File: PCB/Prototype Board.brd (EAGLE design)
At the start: 55.9 x 76.2 mm, 71 parts, among them IC1 SMF05CT1G, J1 USB Type C, J3 Connector, Q1 S8050, Q10 20V/0.2A/8MHz/1.2Ω/1Vth, Q2 20V/0.2A/8MHz/1.2Ω/1Vth, Q3 20V/4.2A/52mΩ/1.4W, Q4 S8050, Q5 20V/0.2A/8MHz/1.2Ω/1Vth, Q6 20V/0.2A/8MHz/1.2Ω/1Vth, Q7 20V/0.2A/8MHz/1.2Ω/1Vth, Q8 20V/0.2A/8MHz/1.2Ω/1Vth, U1 9DoF IMU, U2 MCP73831, U3 ESP-WROOM-32, U5 DWM1000, U7 CH340C

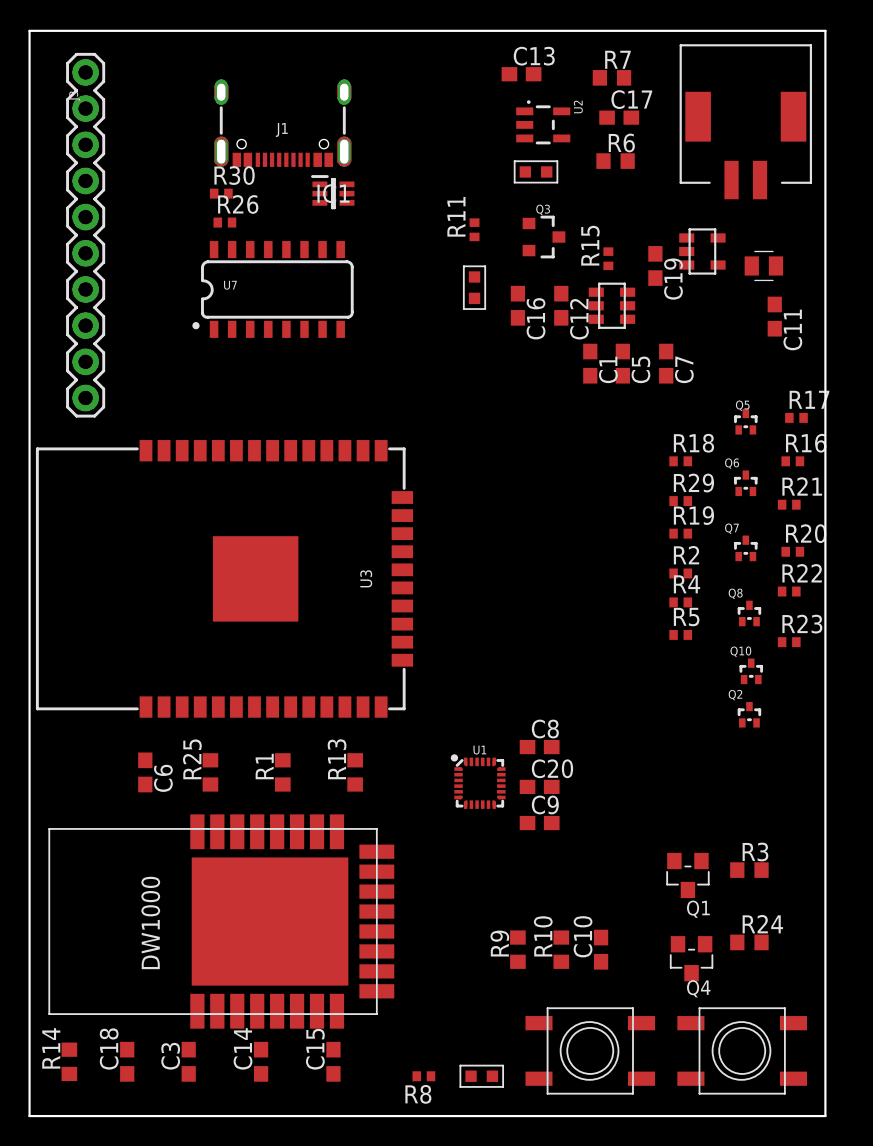
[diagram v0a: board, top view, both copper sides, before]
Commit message: Board Almost Finished
Need to route IO connectors, retouch design rules, clean up connections, etc
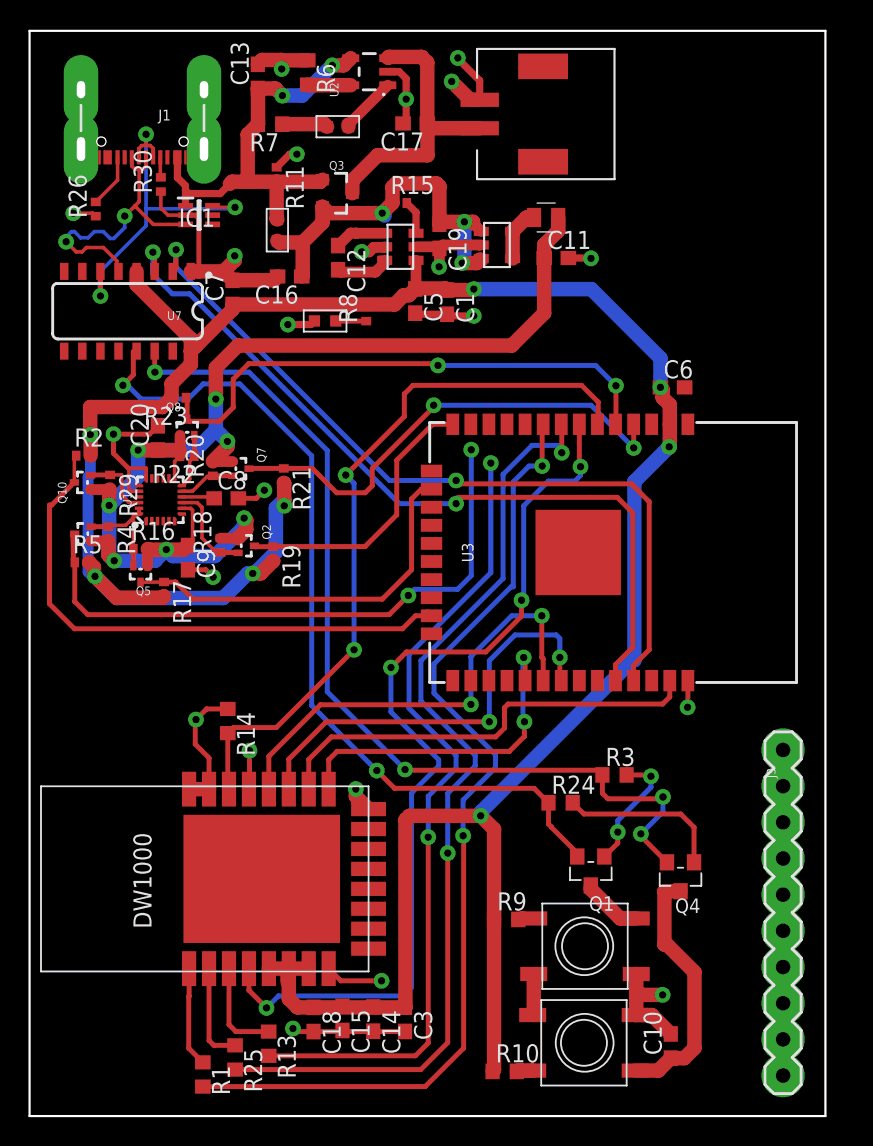
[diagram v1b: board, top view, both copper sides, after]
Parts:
- moved J3 68.3 mm to (52.9, 25.7)
- moved U$9 54.2 mm to (20.8, 55.8), turned to 180 degrees
- moved R8 53.7 mm to (23.6, 56.3), turned to 90 degrees
- moved Q10 49.2 mm to (3.19, 44.5), turned to 90 degrees
- moved Q6 47.2 mm to (3.22, 40.9), turned to 90 degrees
- moved R16 46.2 mm to (7.79, 39.8)
- moved R23 46.2 mm to (10.5, 50.4), turned to 180 degrees
- moved R17 46.0 mm to (9.44, 37.0), turned to 270 degrees
- moved C6 45.8 mm to (45.1, 51.2), turned to 0 degrees
- moved Q5 44.1 mm to (7.79, 37.5), turned to 180 degrees
- moved R22 43.3 mm to (11.1, 46.3), turned to 180 degrees
- moved R2 42.8 mm to (3.78, 46.4)
- moved R5 42.4 mm to (3.68, 38.9)
- moved Q8 41.6 mm to (11.1, 48.9)
- moved R20 41.1 mm to (12.9, 45.5), turned to 90 degrees
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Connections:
- net D+ renamed D_P
- net D- renamed D_N
- net FSYNC/IO33 renamed FSYNC/IO36
- net INT/IO34 renamed INT/IO39
- net RX renamed RX-TX_P
- net TX renamed RX-TX_N
- removed net +3V3: C6.1, R10.1, R9.1, U3.2
- net 3.3V: now also C6.1, R10.1, R9.1, U3.2
- net GND: now also U5.VSS.5
- net IO16: no longer J3.3
- net IO17: no longer J3.4
- net IO2: no longer J3.1
- net IO21: no longer J3.5
- net IO22: no longer J3.6
- net IO25: no longer J3.7
- net IO26: no longer J3.8
- net IO33: no longer Q7.3, R21.1
- net IO34: no longer Q8.3, R23.1
- net IO36: now also Q7.3, R21.1; no longer J3.9
- net IO39: now also Q8.3, R23.1; no longer J3.10
- net IO4: no longer J3.2
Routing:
- net 3.3V: track 0.00 -> 188.2 mm, vias 0 -> 8
- net GND: track 0.00 -> 99.9 mm, vias 0 -> 21
- net 1.8V: track 0.00 -> 88.3 mm, vias 0 -> 7
- net IO33: track 0.00 -> 69.8 mm, vias 0 -> 2
- net IO32: track 0.00 -> 67.8 mm, vias 0 -> 2
- net RTS: track 0.00 -> 66.3 mm, vias 0 -> 4
- net GPIO35: track 0.00 -> 65.7 mm, vias 0 -> 4
- net DTR: track 0.00 -> 60.7 mm, vias 0 -> 2
- net IO27: track 0.00 -> 56.9 mm, vias 0 -> 2
- net RX-TX_P: track 0.00 -> 56.5 mm, vias 0 -> 2
- net RX-TX_N: track 0.00 -> 55.9 mm, vias 0 -> 2
- net IO34: track 0.00 -> 51.2 mm, vias 0 -> 2
- net GPIO14: track 0.00 -> 43.1 mm, vias 0 -> 2
- net GPIO15: track 0.00 -> 39.7 mm
- net IO39: track 0.00 -> 37.9 mm, vias 0 -> 2
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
